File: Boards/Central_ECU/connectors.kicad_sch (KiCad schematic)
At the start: 44 parts, among them J10 Solenoid NANOFIT, J11 DB9 Microfit, J12 RS422 JST, J13 USB_B_Micro, J14 SWD JST PH, J15 UART JST, J2 Extras JST, J3 MICROFIT, J4 Siren MICROFIT, J5 I2CB JST, J6 MICROFIT, J7 I2CA JST, J8 Ignitor JST EH, J9 DB9 MICROFIT, Q4 DMP6023LFG, Q5 DMP6023LFG, SW1 Arm Switch, SW2 On Switch, U7 AZ1117C-5.0, U8 AZ1117C-3.3

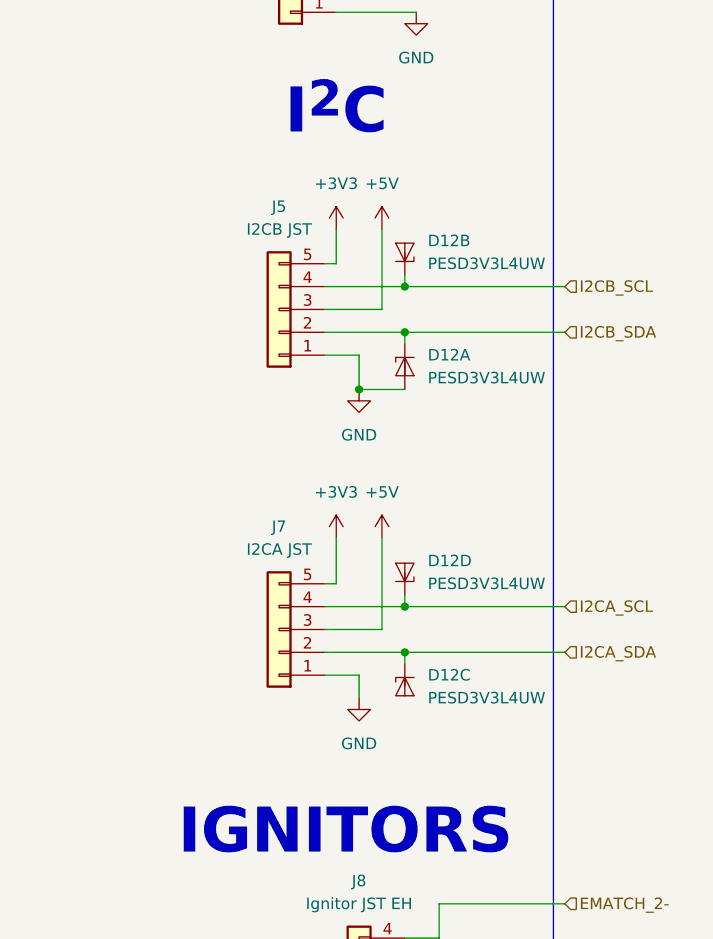
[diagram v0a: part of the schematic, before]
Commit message: Tidy up, will send to Chris
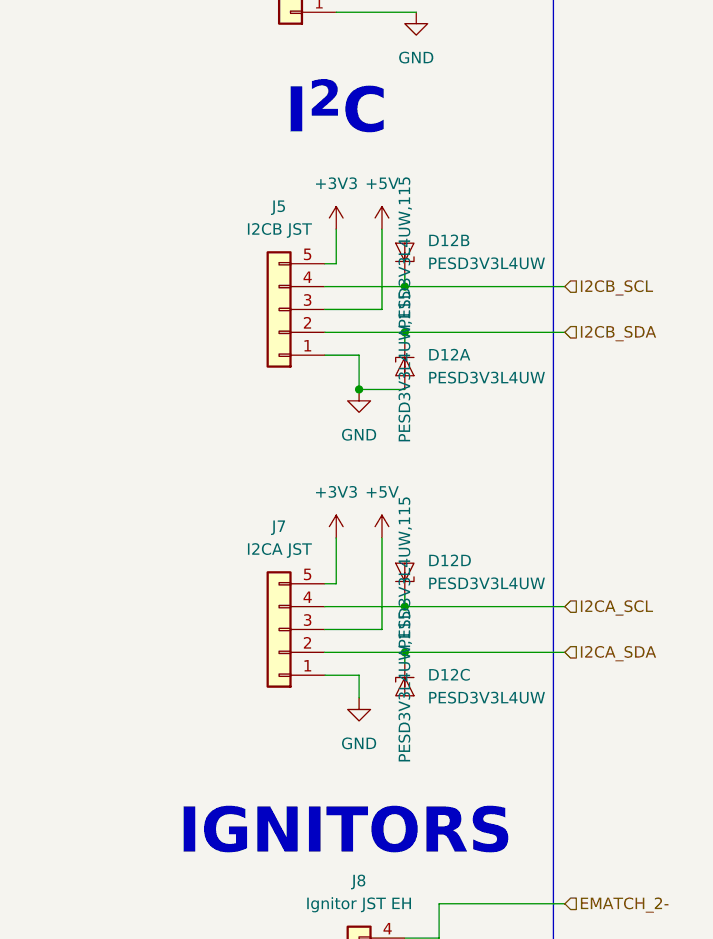
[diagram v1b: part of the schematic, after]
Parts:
- D12: MPN (none) -> PESD3V3L4UW,115
- J6: MPN 430450412 -> 0430450412
